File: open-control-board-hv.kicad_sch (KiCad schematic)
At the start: 20 parts, among them J3 TE 160650-2, J4 TE 160650-2, J5 TE 160650-2, J6 TE 160650-2, J7 TE 160650-2, J8 TE 160650-2, K1 RT314A12, U11 ALDP112, U12 ALDP112, U13 ALDP112

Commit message: Updated with manufacturing data and switched footprint for fastons
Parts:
- J3, J4, J5, J6, J7, J8: footprint 1289:KEYSTONE_1289 -> 624091:TE_62409-1
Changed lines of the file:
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@@
       (effects (font (size 1.27 1.27)))
     )
-    (property "Footprint" "1289:KEYSTONE_1289" (at 200.66 92.71 0)
+    (property "Footprint" "624091:TE_62409-1" (at 200.66 92.71 0)
       (effects (font (size 1.27 1.27)) hide)
     )
@@
       (effects (font (size 1.27 1.27)))
     )
-    (property "Footprint" "1289:KEYSTONE_1289" (at 36.83 85.09 0)
+    (property "Footprint" "624091:TE_62409-1" (at 36.83 85.09 0)
       (effects (font (size 1.27 1.27)) hide)
     )
@@
       (effects (font (size 1.27 1.27)) (justify left))
     )
-    (property "Footprint" "1289:KEYSTONE_1289" (at 82.55 135.89 0)
+    (property "Footprint" "624091:TE_62409-1" (at 82.55 135.89 0)
       (effects (font (size 1.27 1.27)) hide)
     )
@@
       (effects (font (size 1.27 1.27)))
     )
-    (property "Footprint" "1289:KEYSTONE_1289" (at 36.83 93.98 0)
+    (property "Footprint" "624091:TE_62409-1" (at 36.83 93.98 0)
       (effects (font (size 1.27 1.27)) hide)
     )
@@
       (effects (font (size 1.27 1.27)))
     )
-    (property "Footprint" "1289:KEYSTONE_1289" (at 199.39 22.86 0)
+    (property "Footprint" "624091:TE_62409-1" (at 199.39 22.86 0)
       (effects (font (size 1.27 1.27)) hide)
     )
@@
       (effects (font (size 1.27 1.27)))
     )
-    (property "Footprint" "1289:KEYSTONE_1289" (at 201.93 160.02 0)
-      (effects (font (size 1.27 1.27)) hide)
-    )
+    (property "Footprint" "624091:TE_62409-1" (at 201.93 160.02 0)
+      (effects (font (size 1.27 1.27)) hide)
+    )

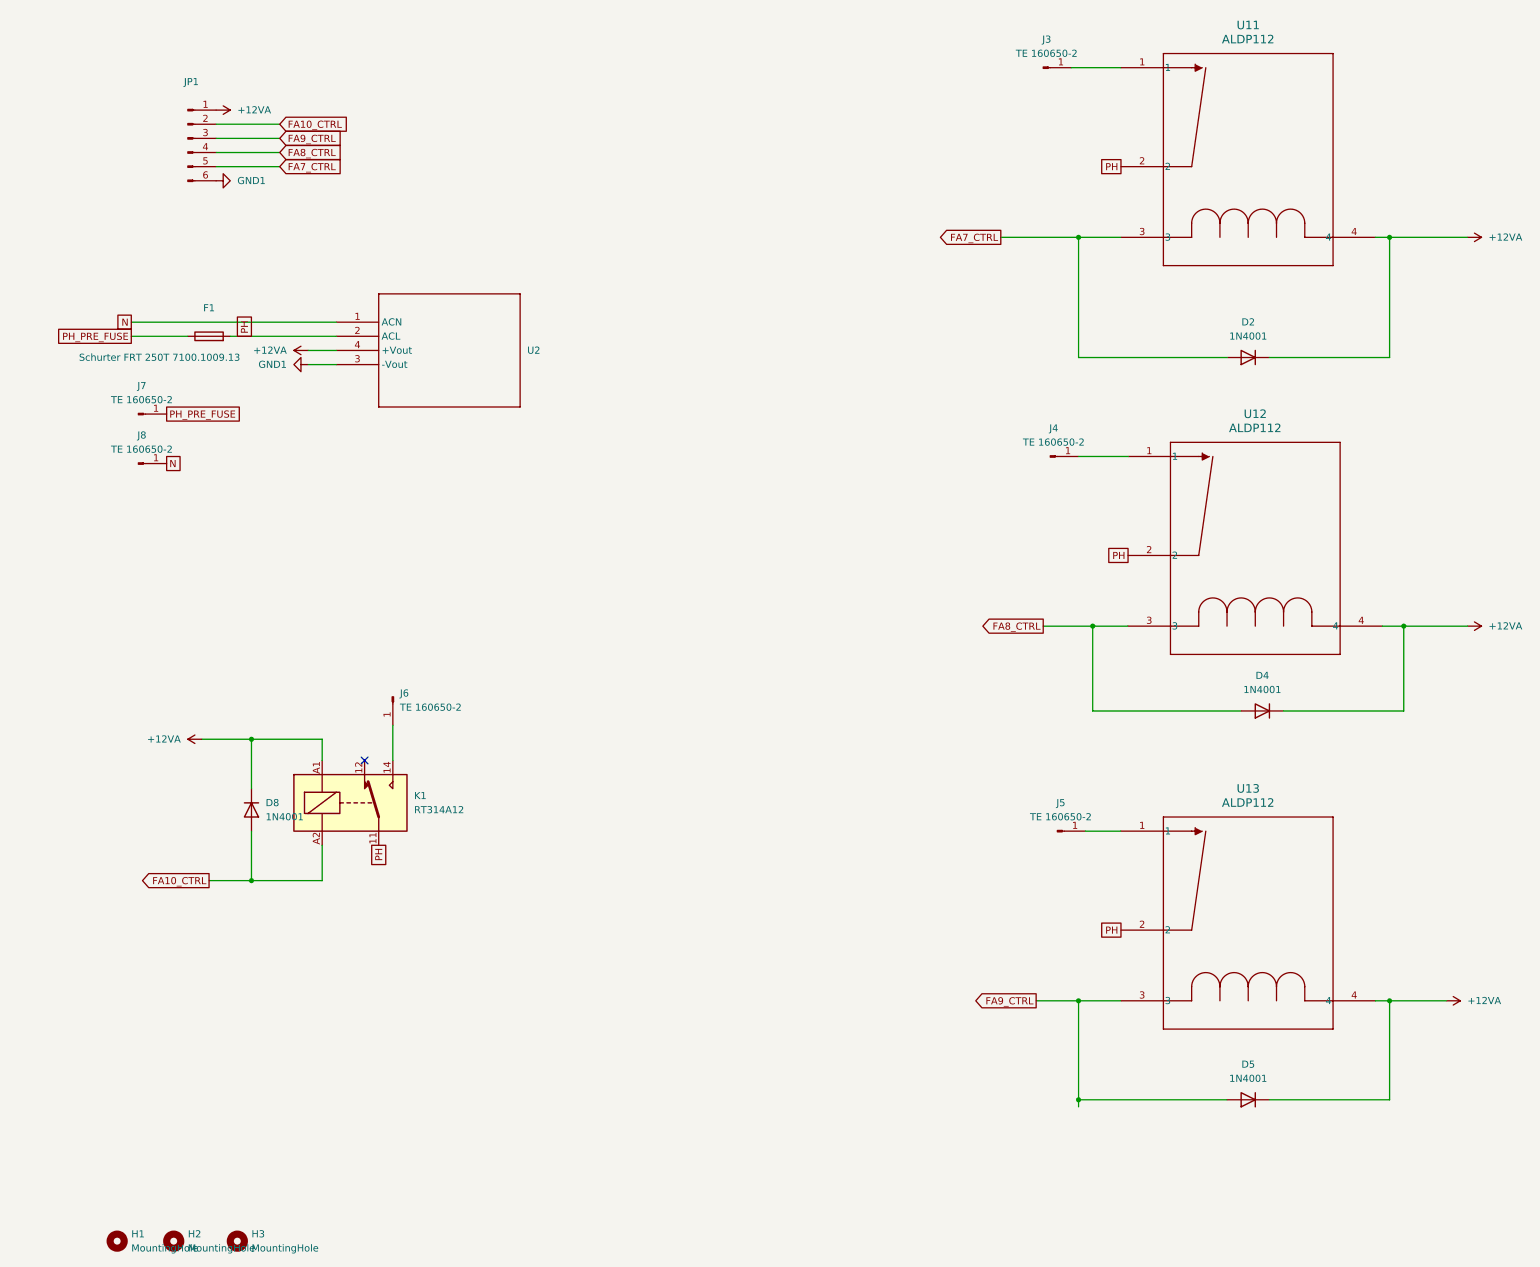
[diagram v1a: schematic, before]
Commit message: Cleanup
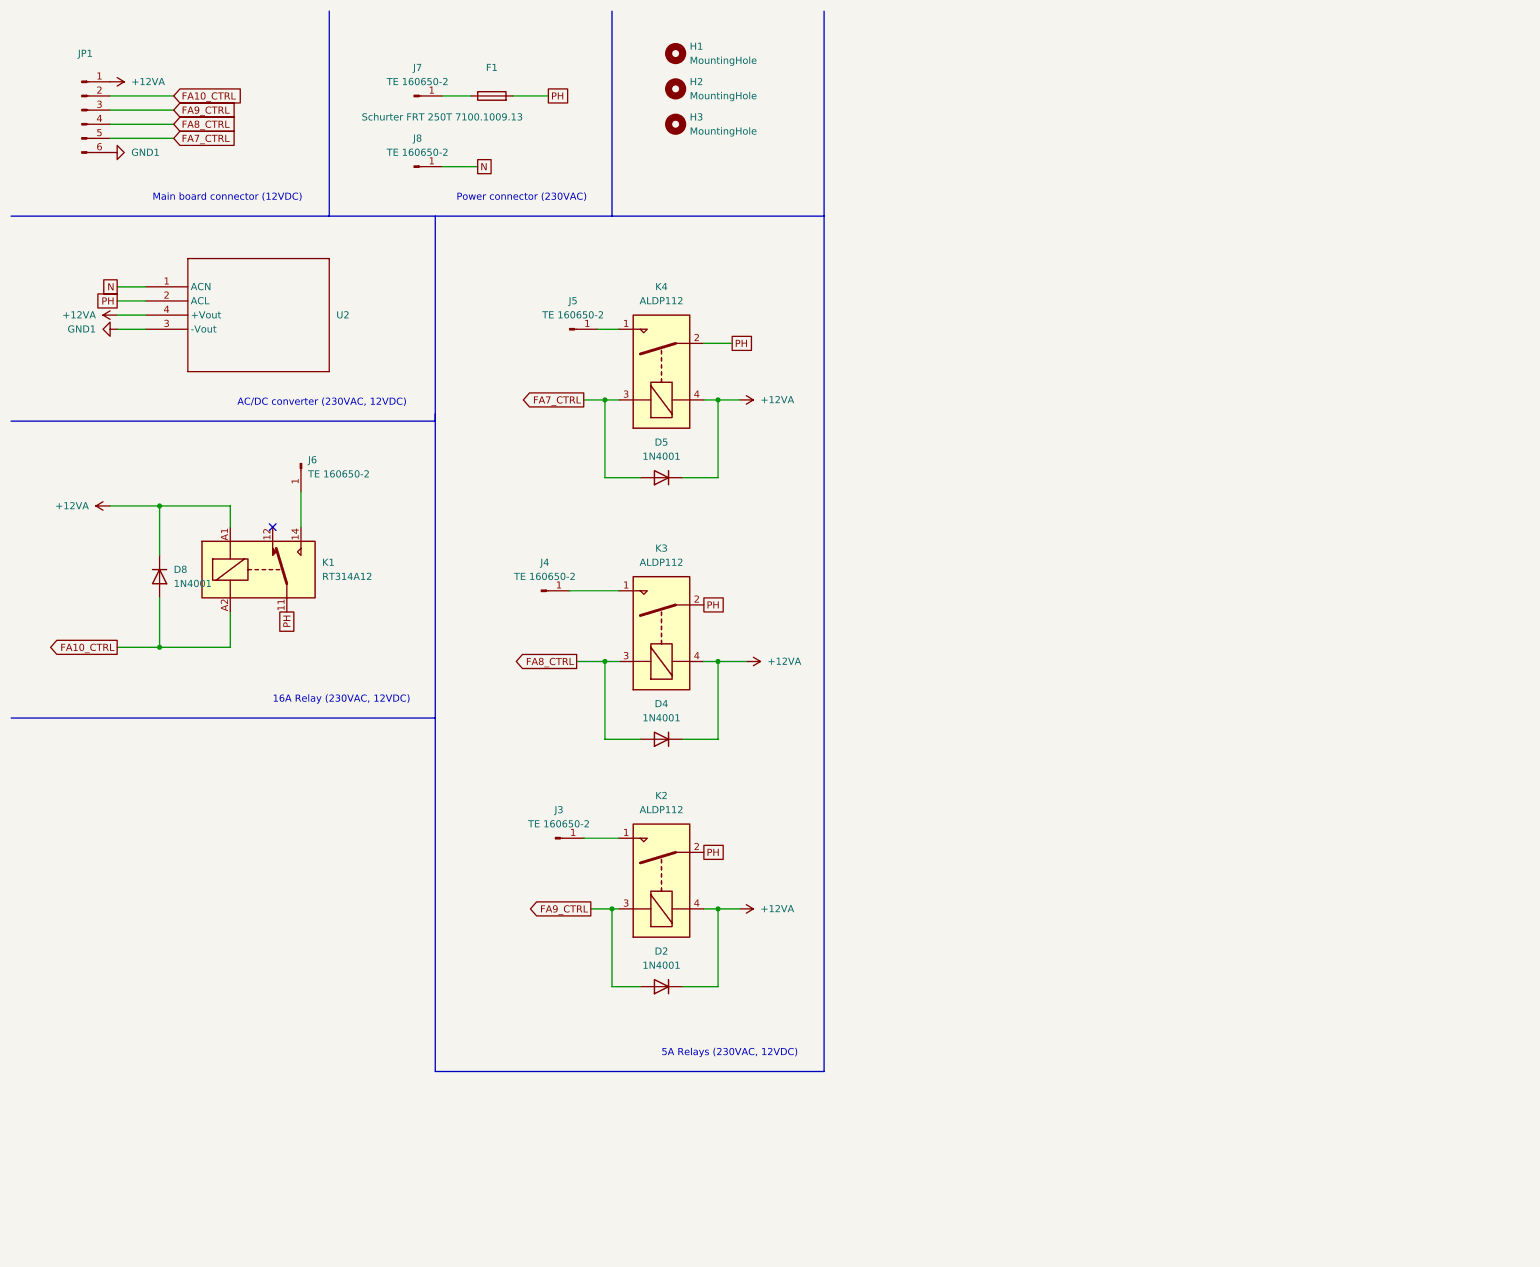
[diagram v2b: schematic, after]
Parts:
- removed U11, U12, U13: ALDP112, ALDP112:PAN_ALD_PAN, symbol ALDP112:ALDP112
- added K2, K3, K4: ALDP112, ALDP112:PAN_ALD_PAN, symbol Relay:Relay_SPST-NO
- D2, D4, D5, D8, U2: Comment (none) -> Hand solder
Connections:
- net +12VA: now also K2.4, K3.4, K4.4
- net FA7_CTRL: now also D5.2 (A), K4.3; no longer D2.2 (A)
- net FA8_CTRL: now also K3.3
- net FA9_CTRL: now also D2.2 (A), K2.3; no longer D5.2 (A)
- net PH: now also K2.2, K3.2, K4.2
- net at J4.1 (Pin_1): now also K3.1
- net at J5.1 (Pin_1): now also K4.1
- net at J3.1 (Pin_1): now also K2.1
- net PH_PRE_FUSE: no longer names the net of F1.1, J7.1 (Pin_1)
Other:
- note added: "16A Relay (230VAC, 12VDC)"
- note added: "5A Relays (230VAC, 12VDC)"
- note added: "AC/DC converter (230VAC, 12VDC)"
- note added: "Main board connector (12VDC)"
- note added: "Power connector (230VAC)"
- moved on the sheet: D4, D8, H1, H2, H3, J4, J6, J7, J8, JP1, K1, U2
